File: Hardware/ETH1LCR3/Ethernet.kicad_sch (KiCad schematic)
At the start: 33 parts, among them U201 LAN8742A, U202 SRV05-4, Y201 NX5032GA-25

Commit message: Hardware
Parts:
- C213, C214: footprint (none) -> Capacitor_SMD:C_1206_3216Metric_Pad1.33x1.80mm_HandSolder
- Y201: footprint (none) -> ETH1LCR3:NX5032GA
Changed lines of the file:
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@@
 			)
 		)
-		(property "Footprint" ""
+		(property "Footprint" "Capacitor_SMD:C_1206_3216Metric_Pad1.33x1.80mm_HandSolder"
 			(at 193.04 117.8052 0)
 			(effects
@@
 			)
 		)
-		(property "Footprint" ""
+		(property "Footprint" "Capacitor_SMD:C_1206_3216Metric_Pad1.33x1.80mm_HandSolder"
 			(at 215.5952 110.49 0)
 			(effects
@@
 			)
 		)
-		(property "Footprint" ""
+		(property "Footprint" "ETH1LCR3:NX5032GA"
 			(at 46.99 118.11 0)
 			(effects

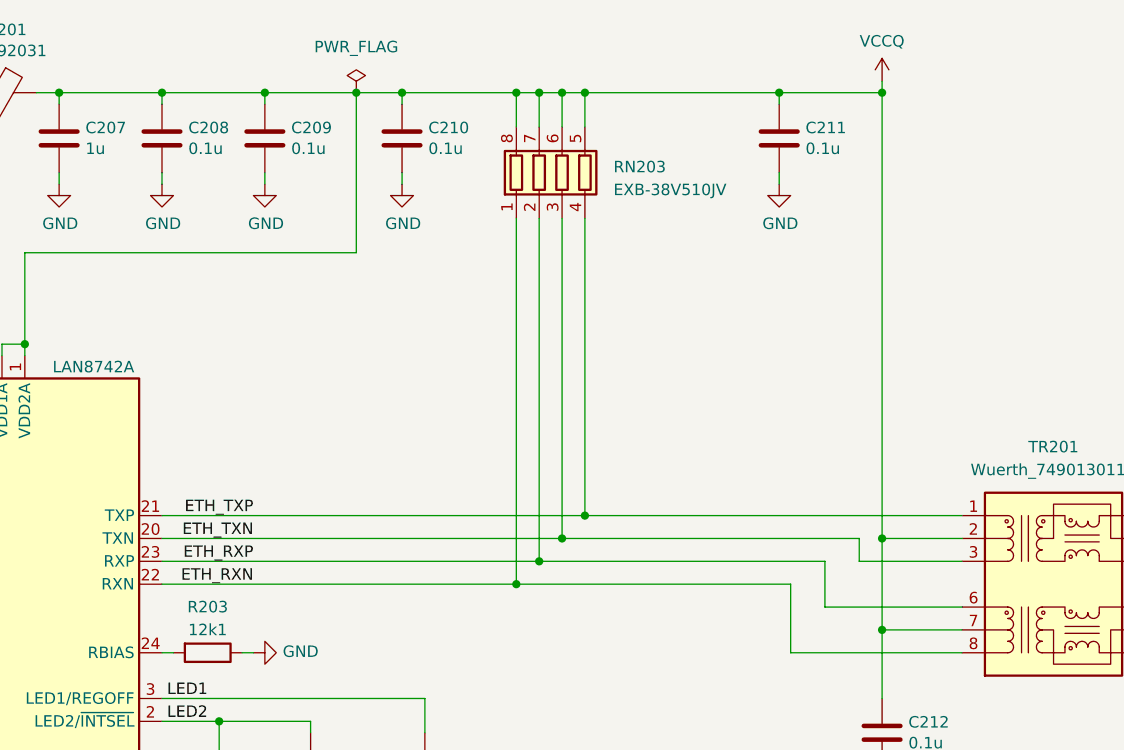
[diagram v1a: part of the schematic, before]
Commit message: PCB layout
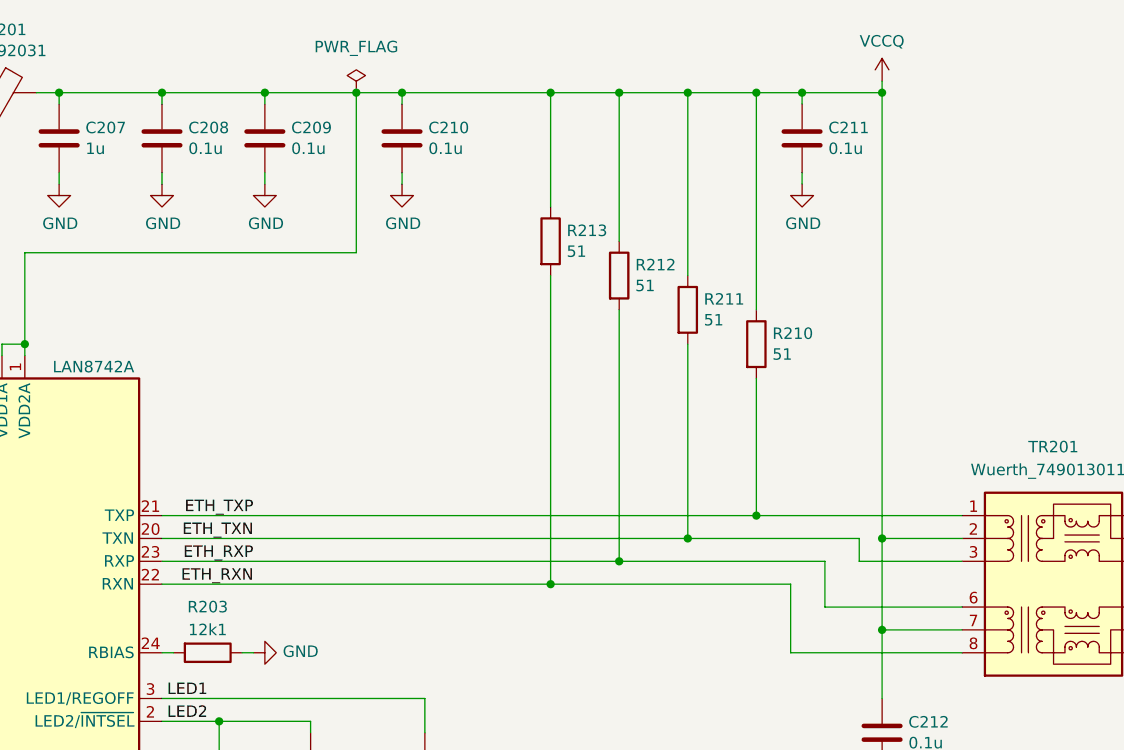
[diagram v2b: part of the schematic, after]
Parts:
- removed RN203: EXB-38V510JV, Resistor_SMD:R_Array_Concave_4x0603, symbol Device:R_Pack04
- added R210, R211, R212, R213: 51, Resistor_SMD:R_0603_1608Metric_Pad0.98x0.95mm_HandSolder, symbol Device:R
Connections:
- net ETH_RXN: now also R213.2
- net ETH_RXP: now also R212.2
- net ETH_TXN: now also R211.2
- net ETH_TXP: now also R210.2
- net VCCQ: now also R210.1, R211.1, R212.1, R213.1
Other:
- moved on the sheet: C211
